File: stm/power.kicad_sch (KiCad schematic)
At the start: 12 parts, among them J3 USB_C_Receptacle_USB2.0_16P, U4 LM1117MP-ADJ

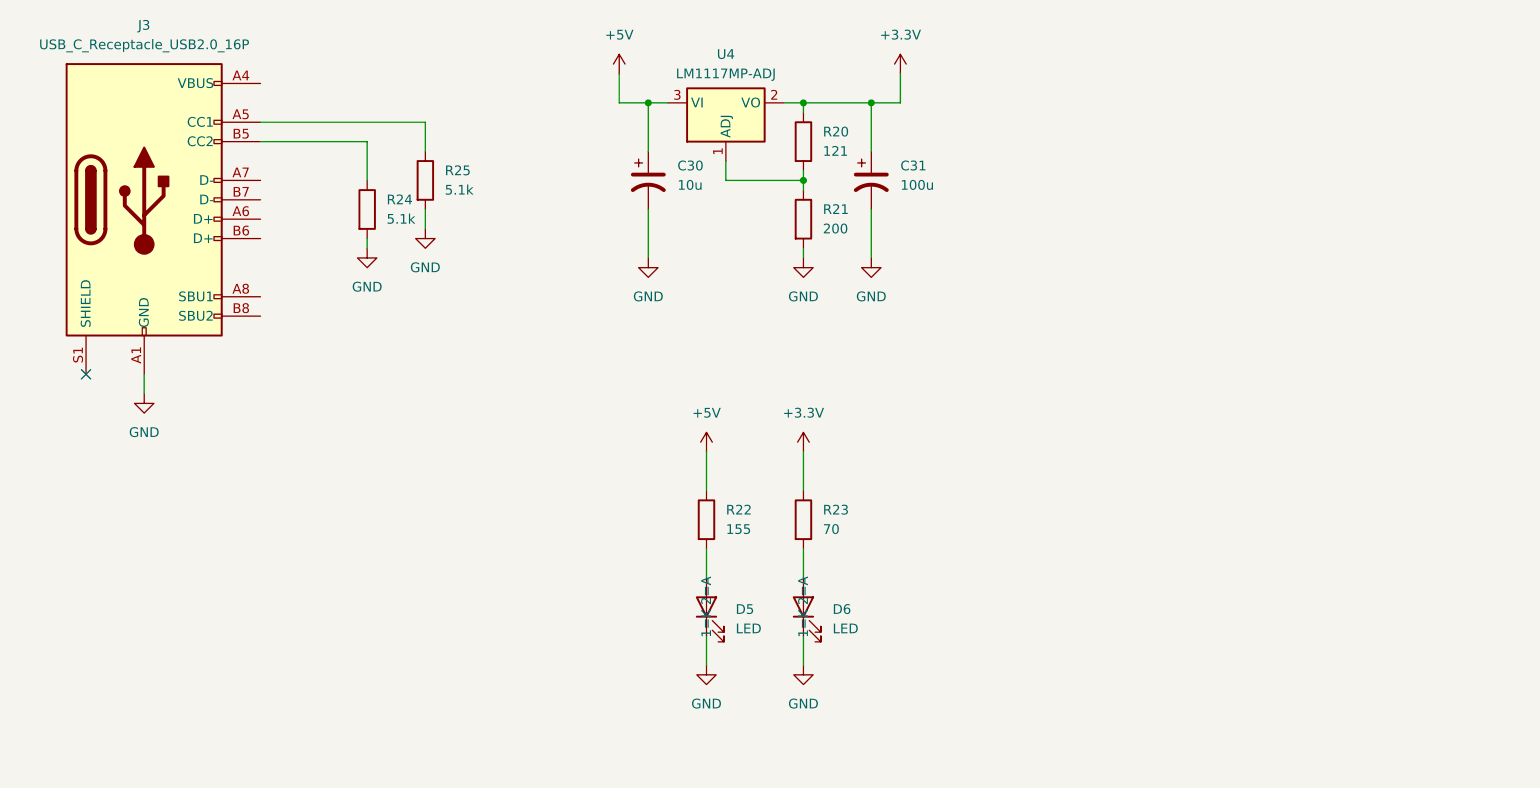
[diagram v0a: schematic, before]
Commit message: usbc power and uart
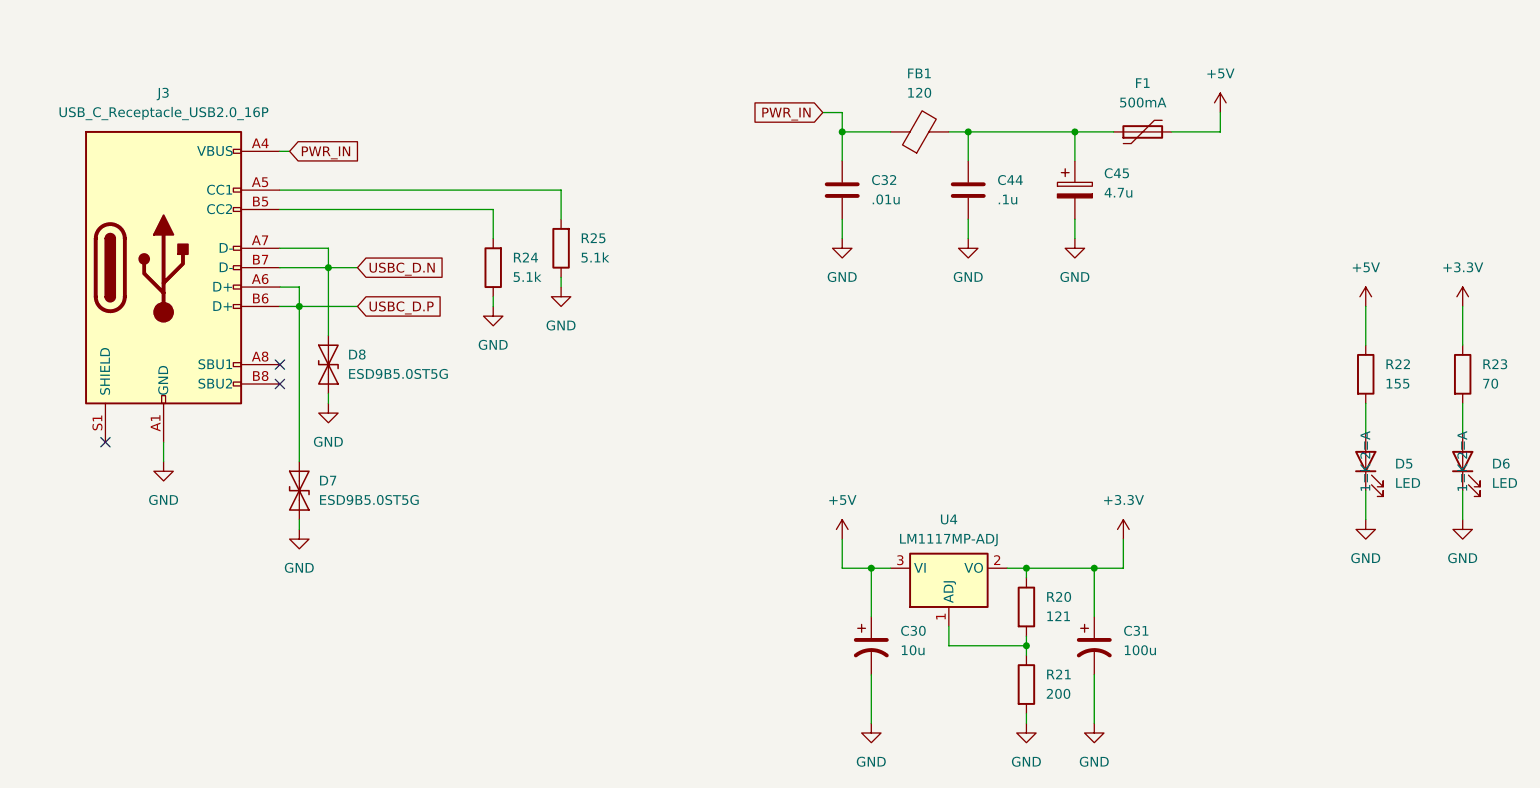
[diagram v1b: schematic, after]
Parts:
- added C32: .01u, Capacitor_SMD:C_0603_1608Metric, symbol Device:C
- added C44: .1u, Capacitor_SMD:C_0603_1608Metric, symbol Device:C
- added C45: 4.7u, Capacitor_SMD:CP_Elec_6.3x7.7, symbol Device:C_Polarized
- added D7, D8: ESD9B5.0ST5G, Diode_SMD:D_SOD-923, symbol Diode:ESD9B5.0ST5G
- added F1: 500mA, Fuse:Fuse_1812_4532Metric, symbol Device:Polyfuse
- added FB1: 120, Inductor_SMD:L_0603_1608Metric, symbol Device:FerriteBead
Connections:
- net +5V: now also F1.2
- net GND: now also R24.1, R25.1, C32.2, C44.2, C45.2, D7.1 (A1), D8.1 (A1); no longer R24.2, R25.2
- net PWR_IN: now reaches J3.A4 (VBUS), J3.A9 (VBUS), J3.B4 (VBUS), J3.B9 (VBUS)
- net PWR_IN: now also C32.1, FB1.1
- net at J3.A5 (CC1): now also R25.2; no longer R25.1
- net USBC_D.P: now reaches J3.A6 (D+)
- net USBC_D.P: now also J3.B6 (D+), D7.2 (A2)
- net USBC_D.N: now reaches J3.A7 (D-)
- net USBC_D.N: now also J3.B7 (D-), D8.2 (A2)
- net at J3.B5 (CC2): now also R24.2; no longer R24.1
- new net: C44.1, C45.1, F1.1, FB1.2
- no-connect marks 1 -> 3
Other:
- moved on the sheet: C30, C31, D5, D6, J3, R20, R21, R22, R23, R24, R25, U4
